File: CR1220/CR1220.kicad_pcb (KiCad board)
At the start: 2 copper layers, 20.3 x 21 mm, 8 parts, among them J1 Conn_01x04

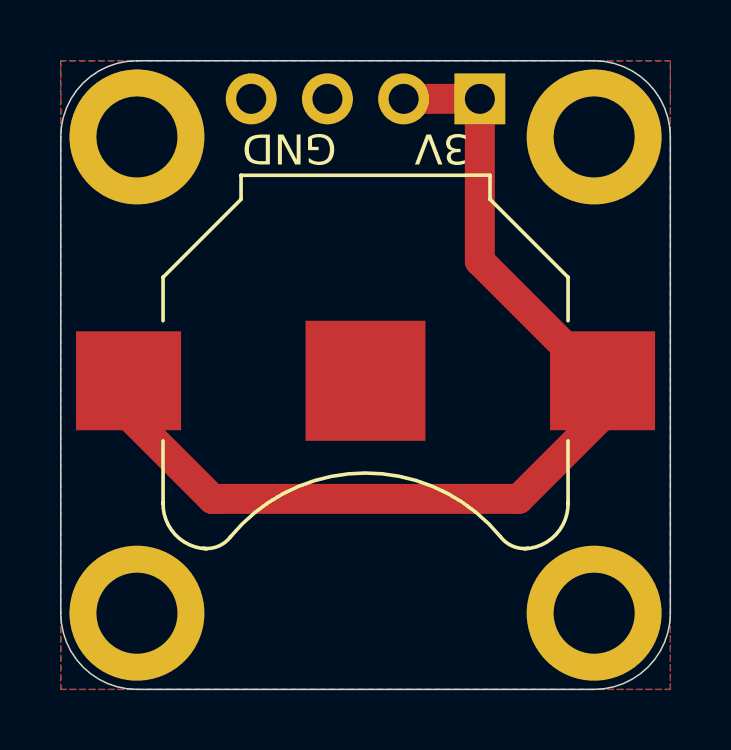
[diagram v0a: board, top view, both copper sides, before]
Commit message: Board Redesign
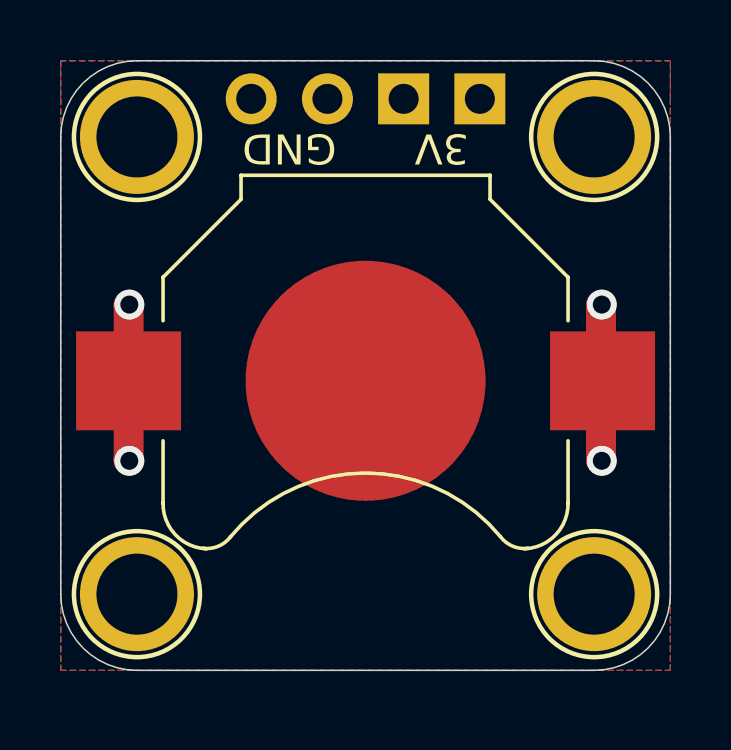
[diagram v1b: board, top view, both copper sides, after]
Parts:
- G***: footprint logo:SirBoard140x44 -> logo:SirBoard112x35
- G***: footprint logo:logo94x134 -> logo:logo76x107
- H1, H2, H3, H4: footprint MountingHole:MountingHole_2.7mm_M2.5_ISO14580_Pad -> SirBoardLibrary:MountingHole_M2.5_SirBoard
- moved H1 15.9 mm to (57.8, 31.4)
- moved H2 15.2 mm to (57.8, 46.6)
- moved G*** 1.78 mm to (65.4, 38.9)
- moved H4 0.63 mm to (73.0, 46.6)
- moved G*** 0.25 mm to (65.4, 44.8)
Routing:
- net +3V0: track 34.1 -> 14.1 mm, vias 0 -> 4
- added copper zone on B.Cu, net +3V0
- removed copper zone on B.Cu, net GND
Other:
- board size 20.3 x 21 mm -> 20.3 x 20.3 mm
- board text added: "www.SirBoard.com"
